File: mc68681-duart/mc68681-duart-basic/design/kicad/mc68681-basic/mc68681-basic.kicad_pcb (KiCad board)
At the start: 4 copper layers, 80 x 110 mm, 36 parts, among them IC1 XR68C681CJTR-F, IC2 74HCT245, IC3 74HCT245, IC4 74HCT245, IC5 74125, IC6 IC6_DECO.PLD, IC7 IC7_UART_.PLD, J1 Conn_02x32_Odd_Even, J2 EXTBUS, J3 UART_A, J4 UART_B, Q1 Crystal

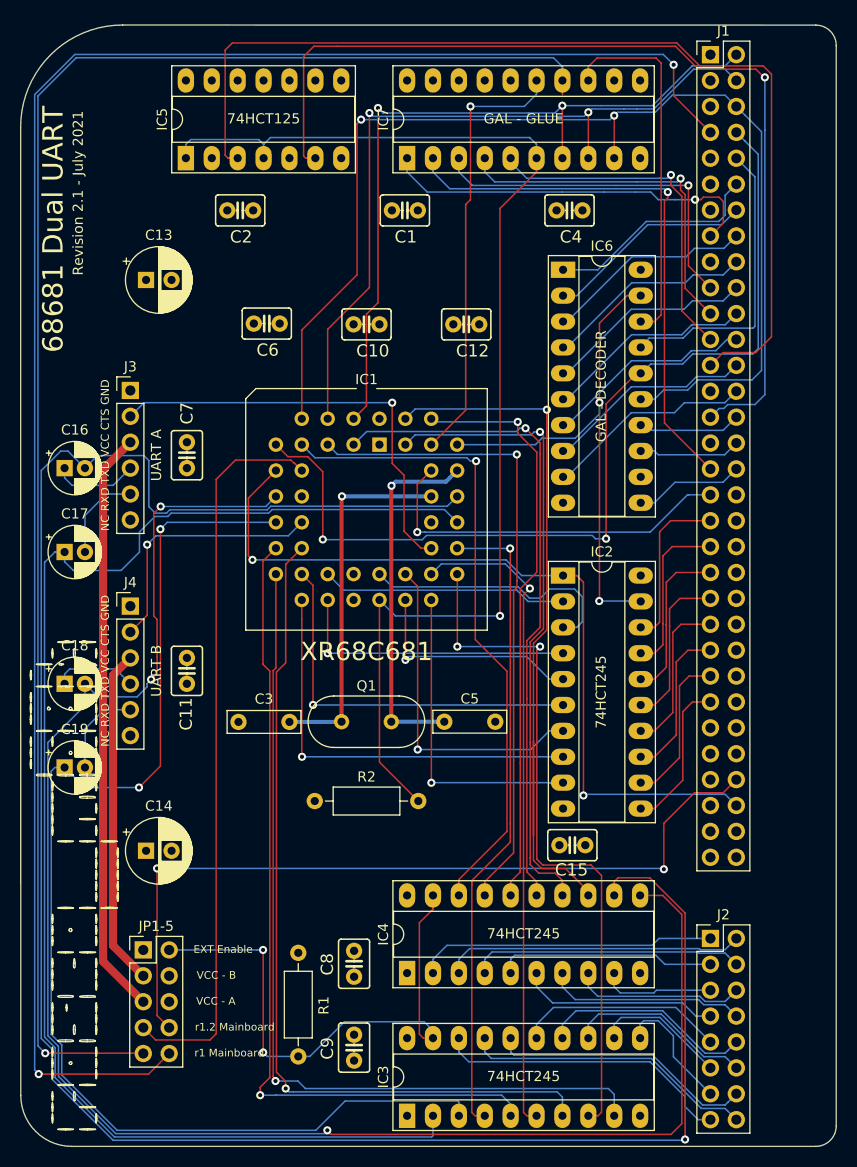
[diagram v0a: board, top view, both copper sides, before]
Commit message: Revert "DUART 2.1"
This reverts commit 27795c8f7bdad45632c07cace90e5a666905ce82.
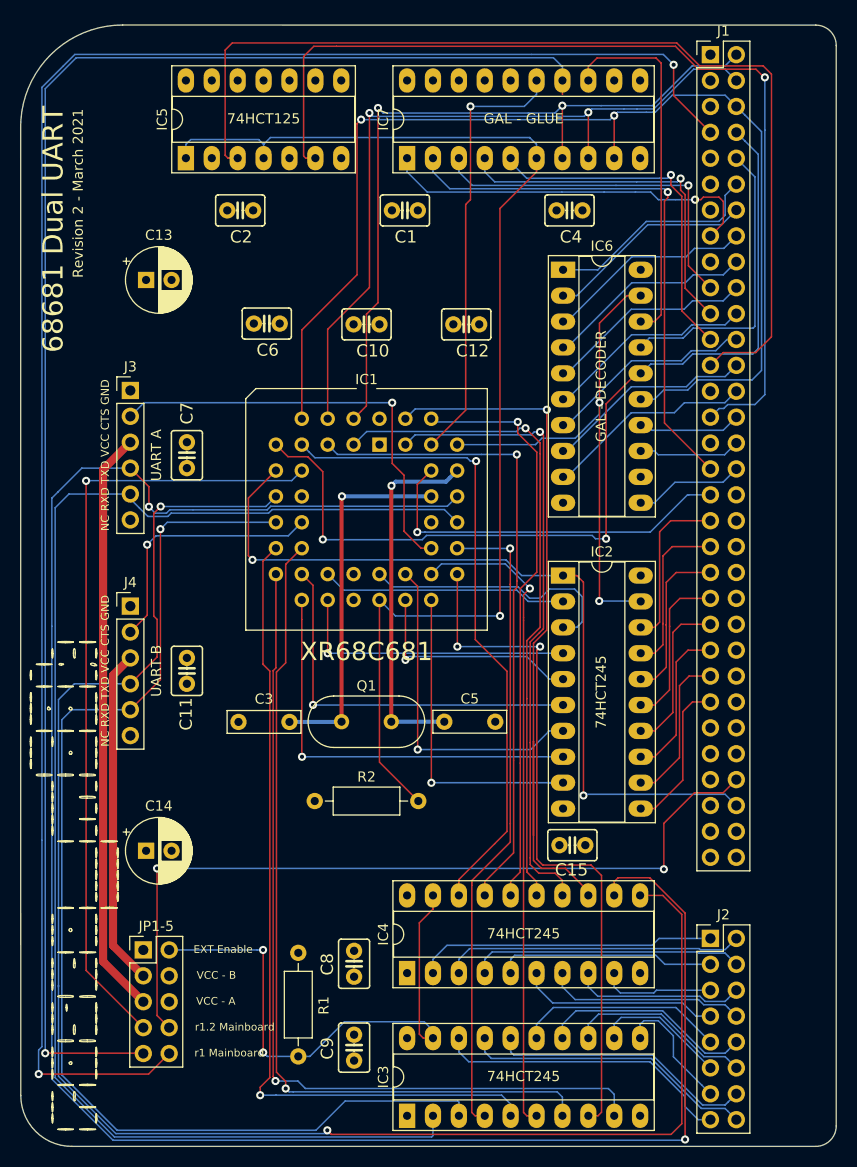
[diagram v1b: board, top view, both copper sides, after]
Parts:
- removed C16, C17, C18, C19: 10uF, Capacitor_THT:CP_Radial_D5.0mm_P2.00mm
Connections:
- J3 pad 4: RXDCA -> RXDA
- J3 pad 5: TXDCA -> TXDA
- J4 pad 4: RXDCB -> RXDB
- J4 pad 5: TXDCB -> TXDB
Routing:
- net TXDCA: track 9.39 -> 0.00 mm
- net TXDCB: track 9.02 -> 0.00 mm
- net RXDCA: track 8.41 -> 0.00 mm
- net RXDCB: track 8.21 -> 0.00 mm
- net RXDA: track 205.3 -> 198.4 mm, vias 1 -> 2
- net UDTACK: track 71.9 -> 77.5 mm, vias 0 -> 1
- net TXDB: track 121.4 -> 116.3 mm, vias 2 -> 1
- net RXDB: track 168.0 -> 165.6 mm, vias 3 -> 2
- net UVPA: track 160.1 -> 159.3 mm
- net TXDA: track 138.2 -> 138.8 mm
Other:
- board text added: "Revision 2 - March 2021"
- board text removed: "Revision 2.1 - July 2021"

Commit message: DUART 2.1
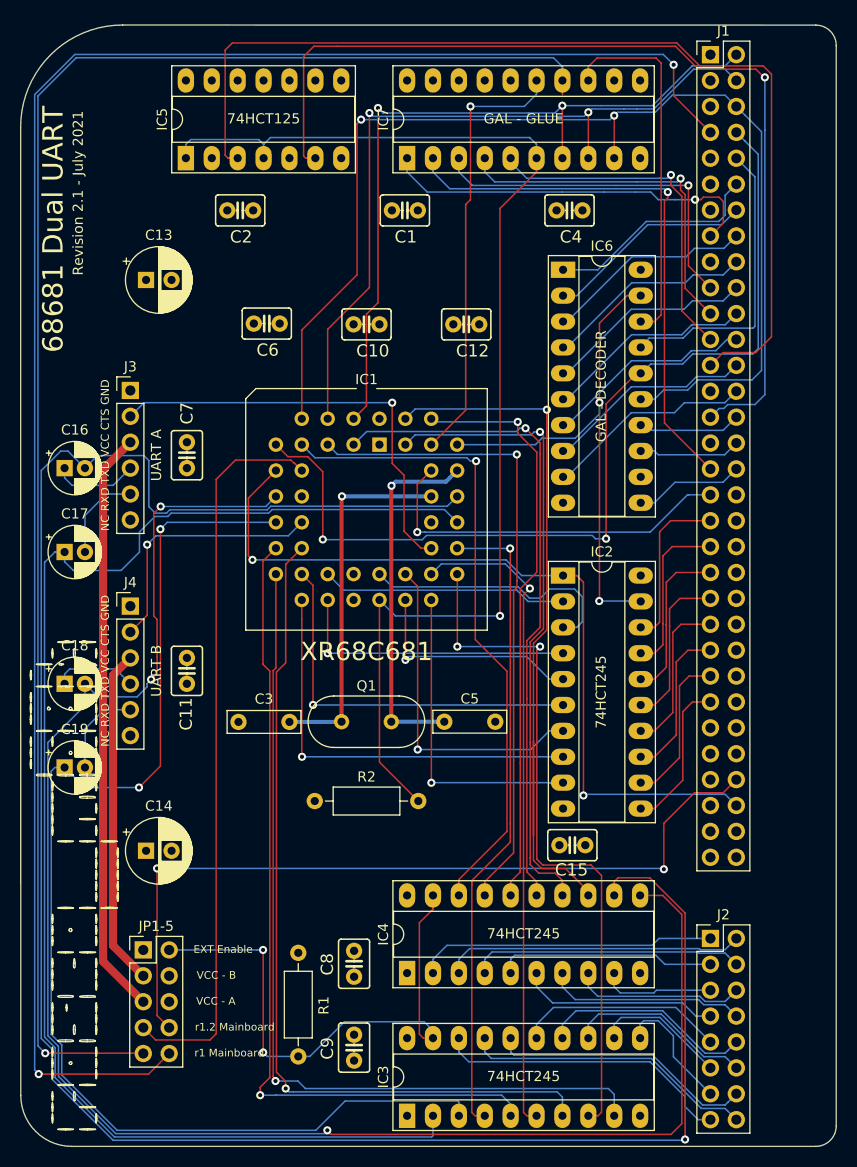
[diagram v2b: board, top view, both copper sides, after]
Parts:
- added C16: 10uF, Capacitor_THT:CP_Radial_D5.0mm_P2.00mm, F.Cu at (55.1, 89.5)
- added C17: 10uF, Capacitor_THT:CP_Radial_D5.0mm_P2.00mm, F.Cu at (55.1, 97.7)
- added C18: 10uF, Capacitor_THT:CP_Radial_D5.0mm_P2.00mm, F.Cu at (55.1, 110.6)
- added C19: 10uF, Capacitor_THT:CP_Radial_D5.0mm_P2.00mm, F.Cu at (55.1, 118.8)
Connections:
- J3 pad 4: RXDA -> RXDCA
- J3 pad 5: TXDA -> TXDCA
- J4 pad 4: RXDB -> RXDCB
- J4 pad 5: TXDB -> TXDCB
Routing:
- net TXDCA: track 0.00 -> 9.39 mm
- net TXDCB: track 0.00 -> 9.02 mm
- net RXDCA: track 0.00 -> 8.41 mm
- net RXDCB: track 0.00 -> 8.21 mm
- net RXDA: track 198.4 -> 205.3 mm, vias 2 -> 1
- net UDTACK: track 77.5 -> 71.9 mm, vias 1 -> 0
- net TXDB: track 116.3 -> 121.4 mm, vias 1 -> 2
- net RXDB: track 165.6 -> 168.0 mm, vias 2 -> 3
- net UVPA: track 159.3 -> 160.1 mm
- net TXDA: track 138.8 -> 138.2 mm
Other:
- board text added: "Revision 2.1 - July 2021"
- board text removed: "Revision 2 - March 2021"
